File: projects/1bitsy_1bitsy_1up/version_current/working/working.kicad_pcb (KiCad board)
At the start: 4 copper layers, 81 x 134 mm, 78 parts, among them CON1 pkl_Micro_SD, J1 pkl_jumper, J2 pkl_jumper, J3 pkl_jumper, J4 pkl_jumper, J6 Jumper_Dual, J7 pkl_JACK_3C1S, P1 PogoPin, Q1 NMOS, SW1 UP, SW10 START, SW11 pkl_SWITCH-SPDT, SW2 Y, SW3 LEFT, SW4 RIGHT, SW5 X, SW6 A, SW7 SELECT, SW8 DOWN, SW9 B, U1 1bitsy-complete-concise, U2 lcd_50pin_logic, U3 lcd_cap_touch_buydisplay, U4 74HC165, U5 74HC165, U6 BQ24075, U7 TPA6135A2, U8 MCP4661-103E/ML

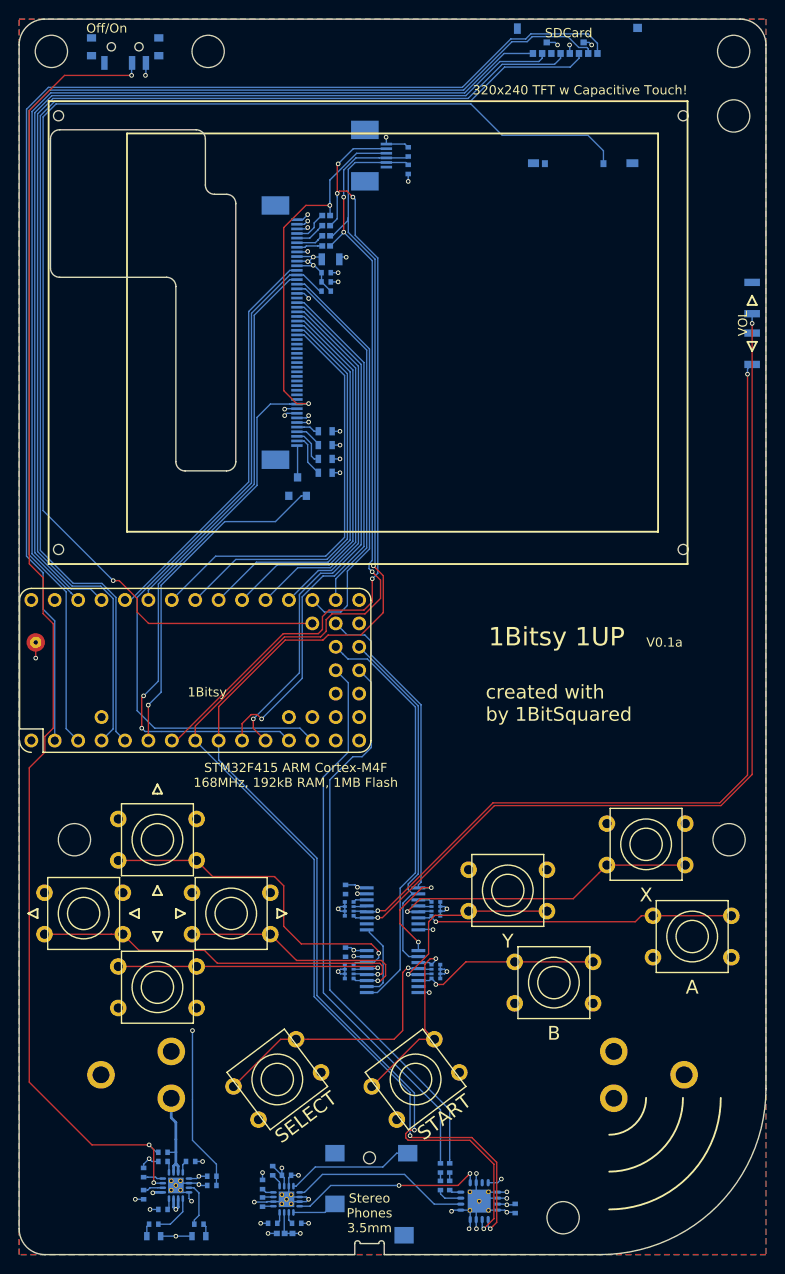
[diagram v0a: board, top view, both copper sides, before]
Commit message: first gitbot try
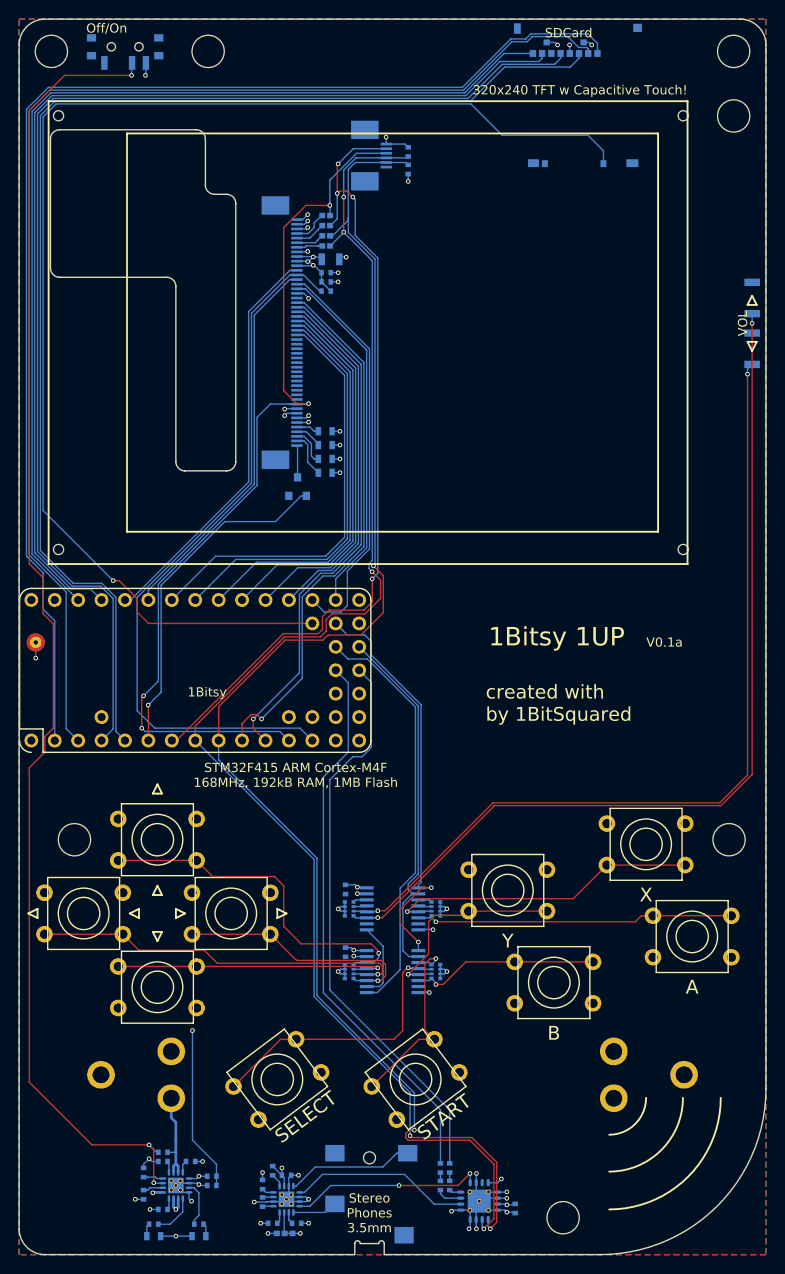
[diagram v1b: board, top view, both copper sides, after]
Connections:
- net /~CHG renamed /~{CHG}
- net /~PGOOD renamed /~{PGOOD}
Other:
- net class Default removed

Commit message: updated all projects from src
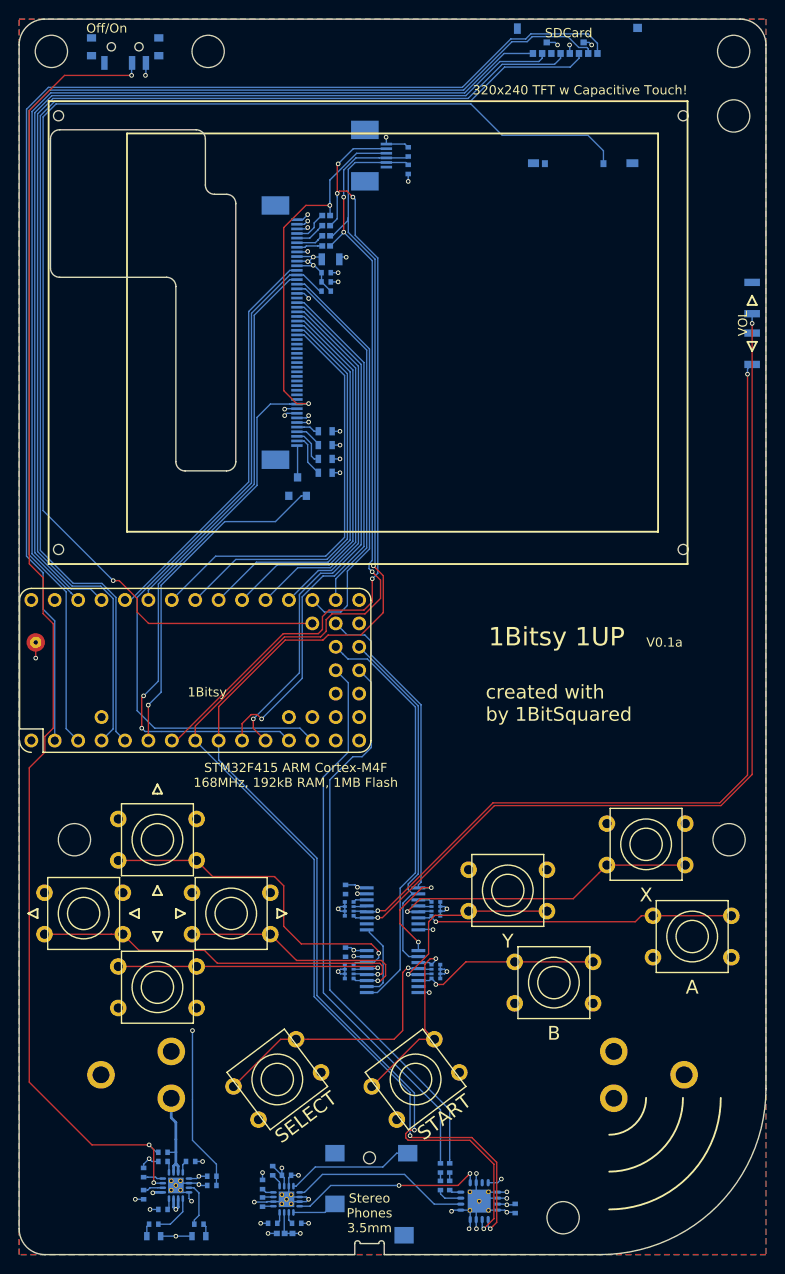
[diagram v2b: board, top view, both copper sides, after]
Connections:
- net /~{CHG} renamed /~CHG
- net /~{PGOOD} renamed /~PGOOD
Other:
- net class Default added: clearance 0.15, trace_width 0.15, via_dia 0.5, via_drill 0.3
